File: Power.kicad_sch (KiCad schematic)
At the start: 3 parts, among them U2 LM2776, U5 LM337L_SO8, U6 LM1117MP-3.3

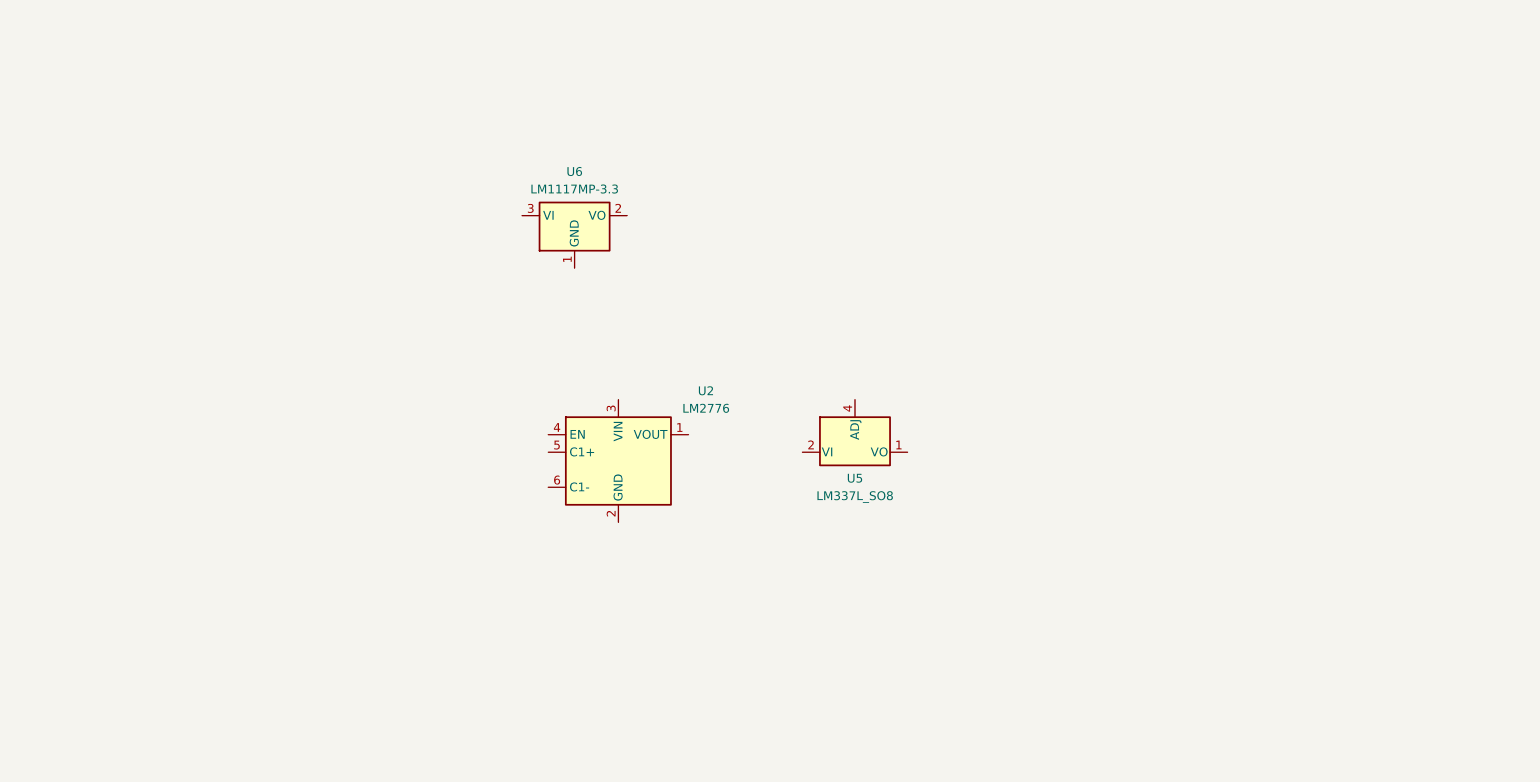
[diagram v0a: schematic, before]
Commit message: dfvdfv
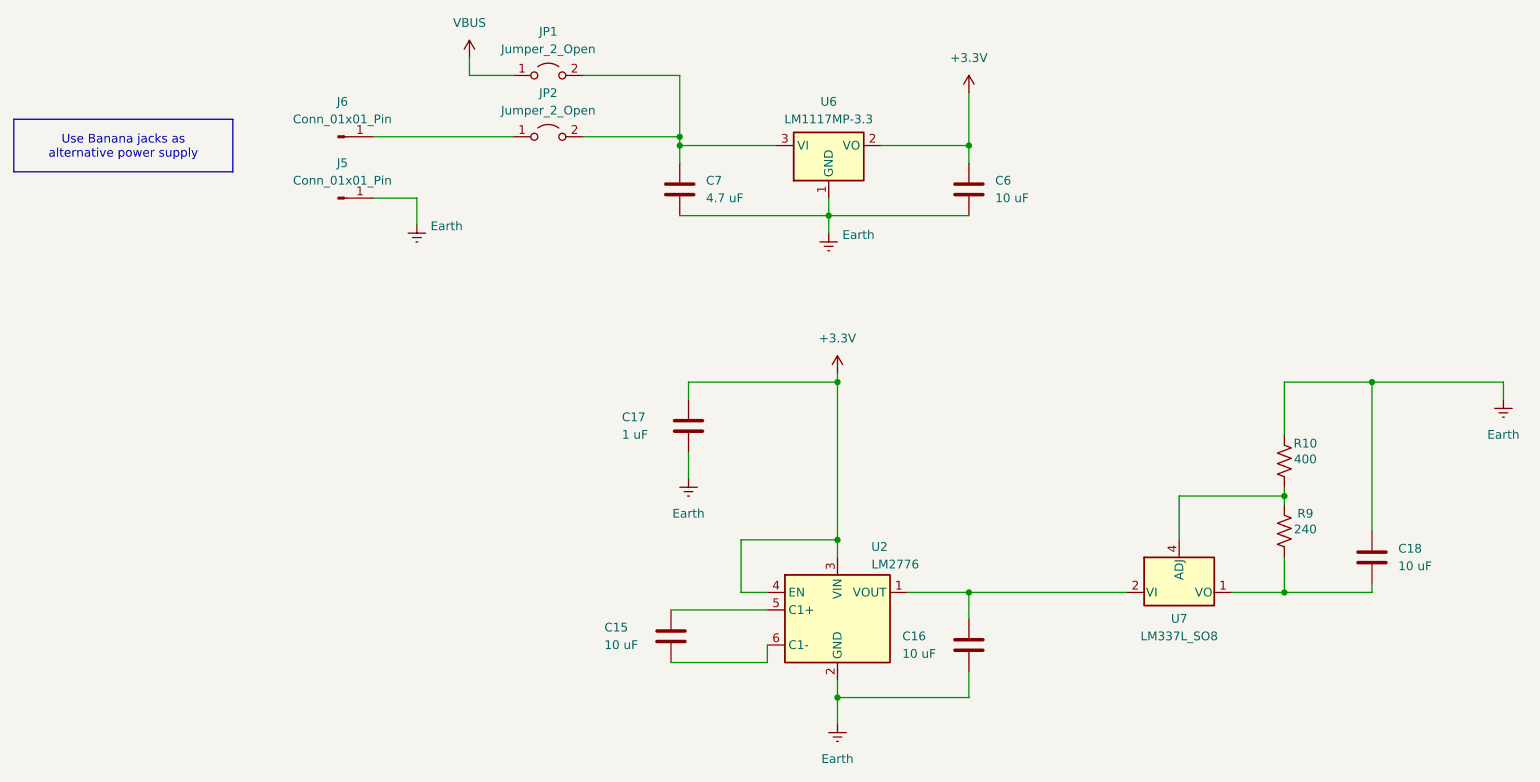
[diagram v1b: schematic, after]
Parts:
- removed U5: LM337L_SO8, Package_SO:SOIC-8_3.9x4.9mm_P1.27mm, symbol Regulator_Linear:LM337L_SO8
- added C15, C16, C18, C6: 10 uF, symbol Device:C
- added C17: 1 uF, symbol Device:C
- added C7: 4.7 uF, symbol Device:C
- added J5, J6: Conn_01x01_Pin, symbol Connector:Conn_01x01_Pin
- added JP1, JP2: Jumper_2_Open, symbol Jumper:Jumper_2_Open
- added R10: 400, symbol Device:R_US
- added R9: 240, symbol Device:R_US
- added U7: LM337L_SO8, Package_SO:SOIC-8_3.9x4.9mm_P1.27mm, symbol Regulator_Linear:LM337L_SO8
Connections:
- net Earth: now reaches U6.1 (GND)
- net Earth: now also U2.2 (GND), C16.2, C17.2, C18.1, C6.2, C7.2, J5.1 (Pin_1), R10.1
- net +3.3V: now reaches U6.2 (VO)
- net +3.3V: now also U2.3 (VIN), U2.4 (EN), C17.1, C6.1
- net at U6.3 (VI): now also C7.1, JP1.2 (B), JP2.2 (B)
- net at U2.1 (VOUT): now also C16.1, U7.2 (VI), U7.3 (VI), U7.6 (VI), U7.7 (VI)
- net at U2.5 (C1+): now also C15.1
- net at U2.6 (C1-): now also C15.2
- new net: J6.1 (Pin_1), JP2.1 (A)
- new net: C18.2, R9.2, U7.1 (VO)
- new net: R10.2, R9.1, U7.4 (ADJ)
- new net VBUS: JP1.1 (A)
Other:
- moved on the sheet: U2, U6
